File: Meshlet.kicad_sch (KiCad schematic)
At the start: 90 parts, among them J1 Ext. Notif. Header, J10 STEMMA QT I2C, J11 GPIO Exp., J2 USB_C_Receptacle_USB2.0_16P, J3 Ext. Power Header, J4 Batt. Header (JST-PH 2.0), J5 SWD, J6 Batt. Header (Picoblade 1.25), J7 GPS Header, J8 User Btn Header, J9 Power Switch, Q1 AO3400A, SW1 BOOTSEL, SW2 USER, SW3 RST, U1 W25Q32JVZP, U2 XC6206PxxxMR, U3 RP2350_60QFN, U4 INA3221, U5 BME280, U6 Wio-SX1262, U7 USBLC6-2SC6, U8 BQ24074RGT, Y1 12.000MHz

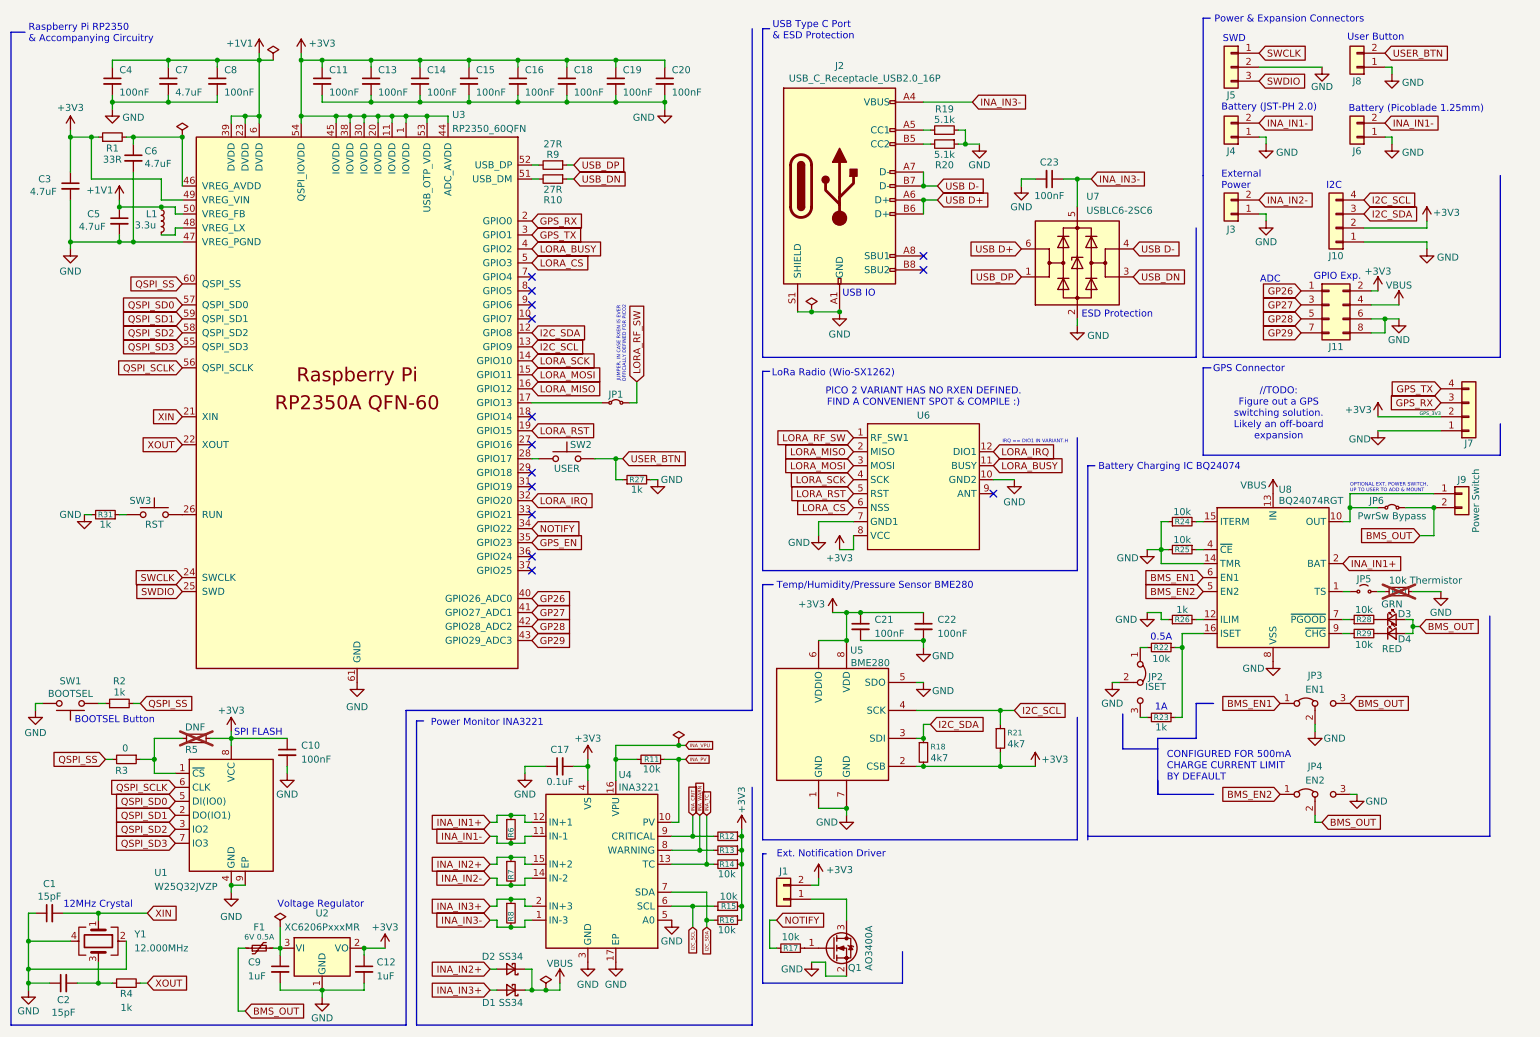
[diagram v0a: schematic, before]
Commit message: PCB routing like 99% done oops
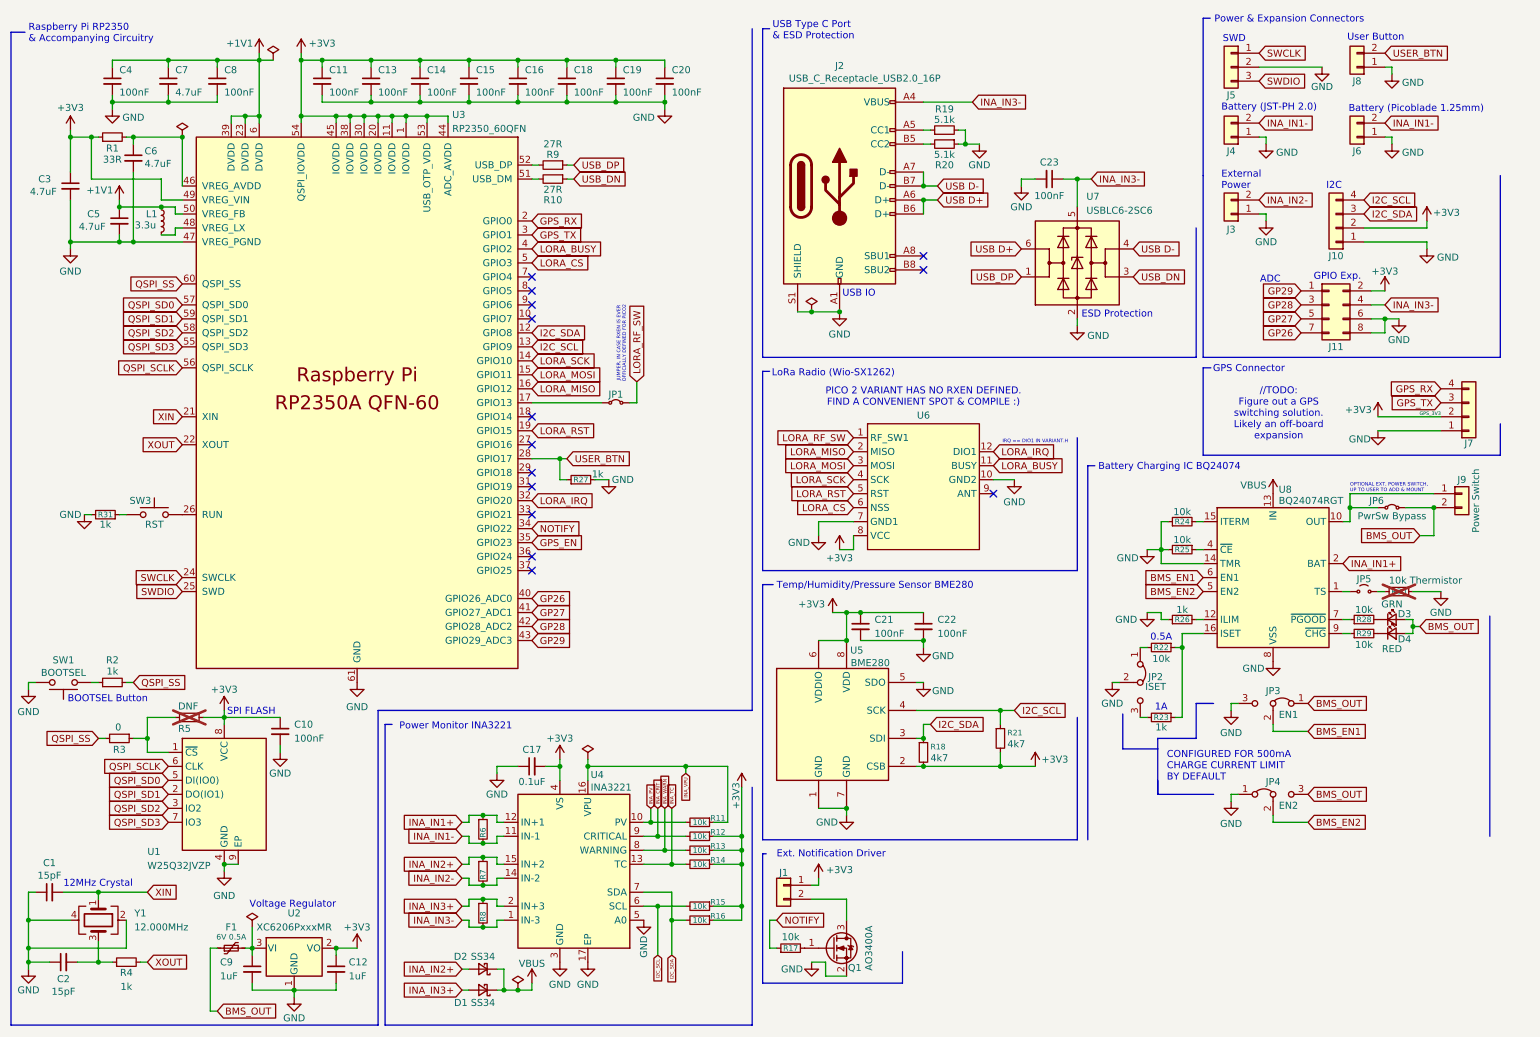
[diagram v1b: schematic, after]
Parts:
- removed SW2: USER, Button_Switch_SMD:SW_Push_1P1T_XKB_TS-1187A, symbol Switch:SW_Push
- J11: footprint Connector_PinHeader_2.00mm:PinHeader_2x04_P2.00mm_Vertical -> Connector_PinHeader_1.27mm:PinHeader_2x04_P1.27mm_Vertical
- J5: footprint Connector_JST:JST_SH_SM02B-SRSS-TB_1x02-1MP_P1.00mm_Horizontal -> Connector_JST:JST_SH_SM03B-SRSS-TB_1x03-1MP_P1.00mm_Horizontal
- J7: footprint Connector_PinHeader_2.54mm:PinHeader_1x04_P2.54mm_Vertical -> Connector_PinHeader_1.27mm:PinHeader_1x04_P1.27mm_Vertical
- J8: footprint Connector_JST:JST_PH_S2B-PH-SM4-TB_1x02-1MP_P2.00mm_Horizontal -> Connector_PinHeader_1.27mm:PinHeader_1x02_P1.27mm_Vertical
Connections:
- net +3V3: now also J1.1 (Pin_1), R15.1; no longer J1.2 (Pin_2), R15.2
- net BMS_EN1: now also JP3.2 (C); no longer JP3.1 (A)
- net BMS_EN2: now also JP4.2 (C); no longer JP4.1 (A)
- net BMS_OUT: now also JP3.1 (A), JP4.3 (B); no longer JP3.3 (B), JP4.2 (C)
- net GND: now also JP3.3 (B), JP4.1 (A); no longer JP3.2 (C), JP4.3 (B)
- net GP26: now also J11.7 (Pin_7); no longer J11.1 (Pin_1)
- net GP27: now also J11.5 (Pin_5); no longer J11.3 (Pin_3)
- net GP28: now also J11.3 (Pin_3); no longer J11.5 (Pin_5)
- net GP29: now also J11.1 (Pin_1); no longer J11.7 (Pin_7)
- net GPS_RX: now also J7.4 (Pin_4); no longer J7.3 (Pin_3)
- net GPS_TX: now also J7.3 (Pin_3); no longer J7.4 (Pin_4)
- net I2C_SCL: now also R15.2; no longer R15.1
- net INA_IN3-: now also J11.4 (Pin_4)
- net USER_BTN: now also U3.28 (GPIO17)
- net VBUS: no longer J11.4 (Pin_4)
- net at Q1.3 (D): now also J1.2 (Pin_2); no longer J1.1 (Pin_1)
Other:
- moved on the sheet: C1, C10, C12, C17, C2, C9, D1, D2, F1, J1, JP3, JP4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
